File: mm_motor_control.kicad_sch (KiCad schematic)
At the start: 0 parts

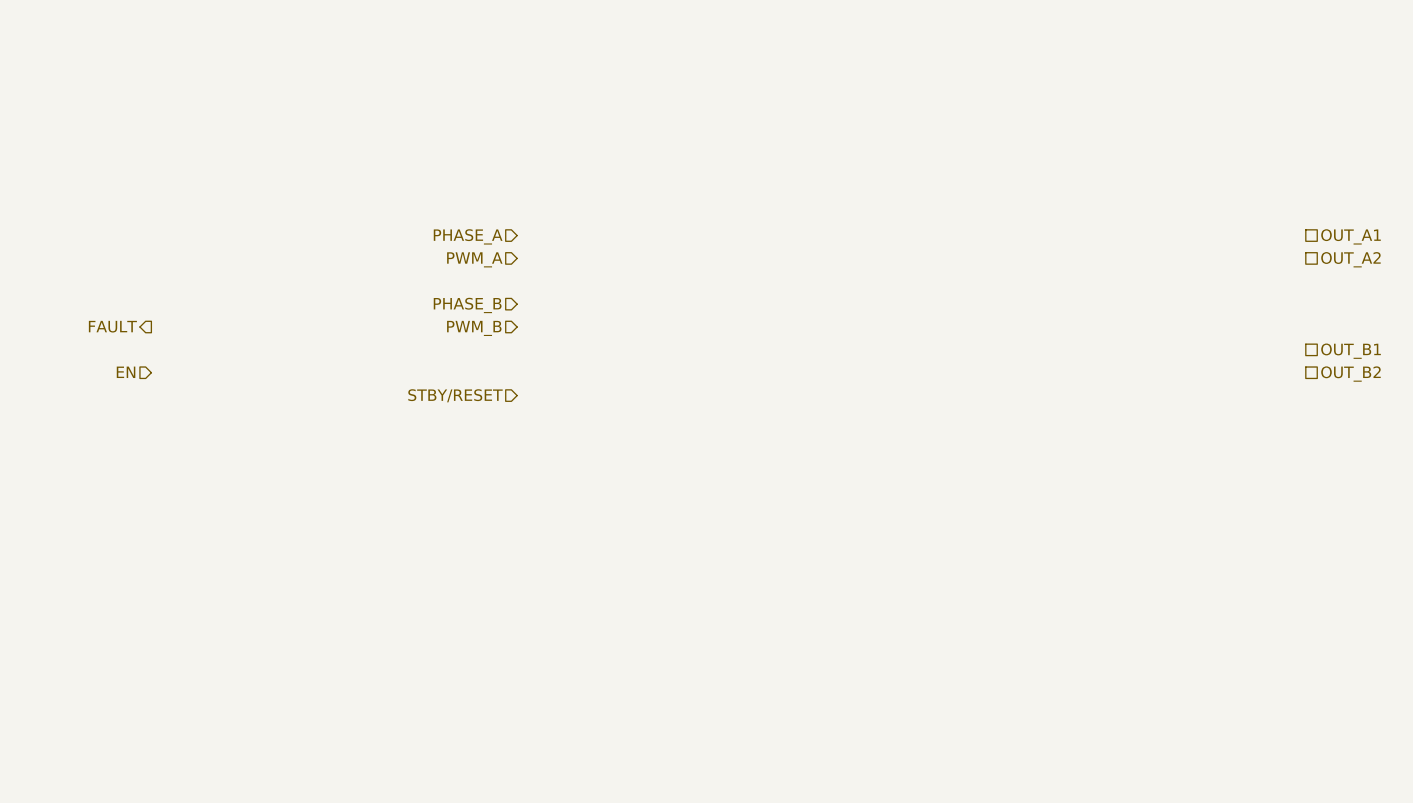
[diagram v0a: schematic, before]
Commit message: tp2
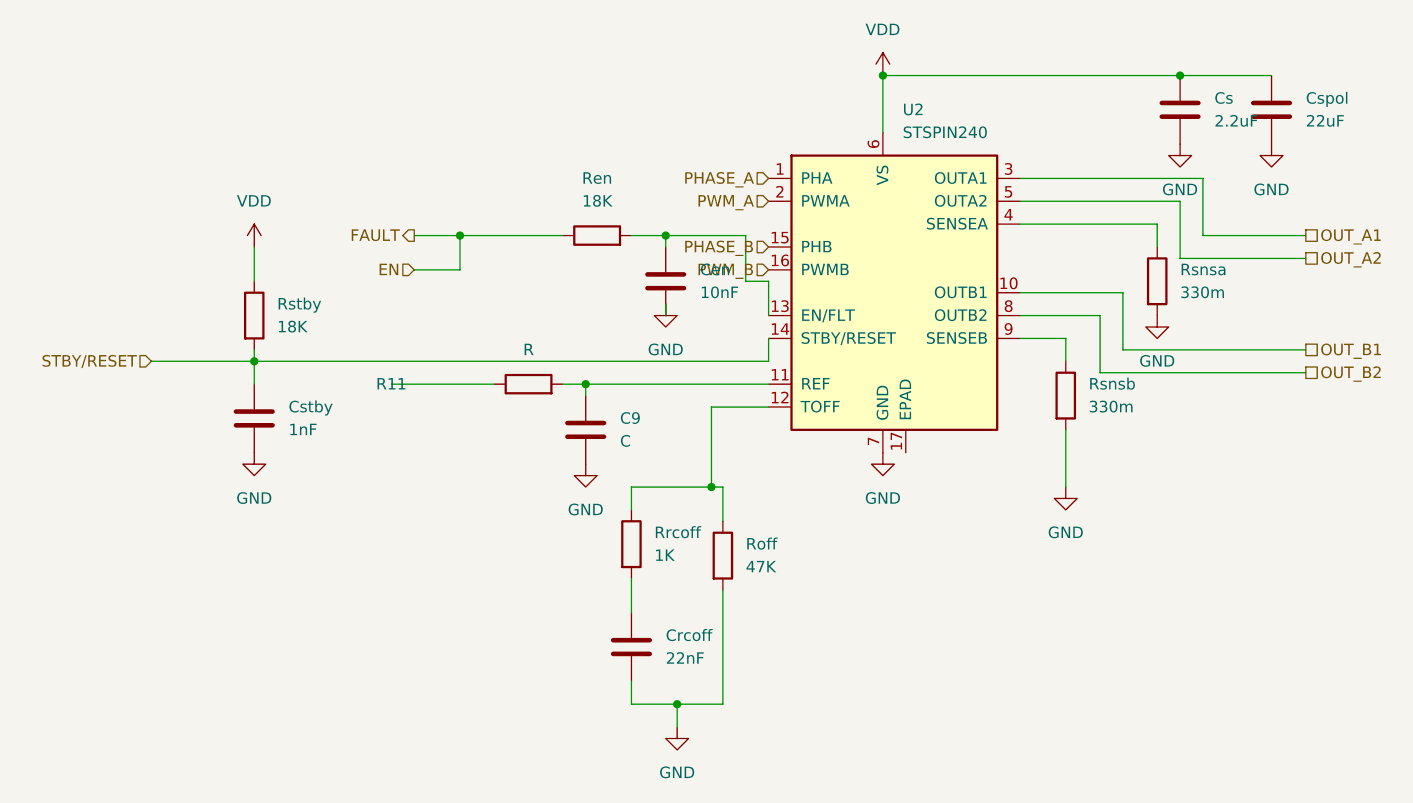
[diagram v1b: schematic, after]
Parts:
- added C9: C, symbol Device:C
- added Cen: 10nF, symbol Device:C
- added Crcoff: 22nF, symbol Device:C
- added Cs: 2.2uF, symbol Device:C
- added Cspol: 22uF, symbol Device:C
- added Cstby: 1nF, symbol Device:C
- added R11: R, symbol Device:R
- added Ren, Rstby: 18K, symbol Device:R
- added Roff: 47K, symbol Device:R
- added Rrcoff: 1K, symbol Device:R
- added Rsnsa, Rsnsb: 330m, symbol Device:R
- added U2: STSPIN240, Package_DFN_QFN:VQFN-16-1EP_3x3mm_P0.5mm_EP1.8x1.8mm, symbol Driver_Motor:STSPIN240
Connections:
- net EN: now also Ren.1
- net OUT_A1: now also U2.3 (OUTA1)
- net OUT_A2: now also U2.5 (OUTA2)
- net OUT_B1: now also U2.10 (OUTB1)
- net OUT_B2: now also U2.8 (OUTB2)
- net PHASE_A: now also U2.1 (PHA)
- net PHASE_B: now also U2.15 (PHB)
- net PWM_A: now also U2.2 (PWMA)
- net PWM_B: now also U2.16 (PWMB)
- net STBY/RESET: now also Cstby.1, Rstby.2, U2.14 (STBY/RESET)
- new net: Crcoff.1, Rrcoff.2
- new net: Roff.1, Rrcoff.1, U2.12 (TOFF)
- new net: Cen.1, Ren.2, U2.13 (EN/FLT)
- new net: C9.1, R11.2, U2.11 (REF)
- new net: Rsnsb.1, U2.9 (SENSEB)
- new net: Rsnsa.1, U2.4 (SENSEA)
- new net GND: C9.2, Cen.2, Crcoff.2, Cs.1, Cspol.1, Cstby.2, Roff.2, Rsnsa.2, Rsnsb.2, U2.7 (GND)
- new net VDD: Cs.2, Cspol.2, Rstby.1, U2.6 (VS)
